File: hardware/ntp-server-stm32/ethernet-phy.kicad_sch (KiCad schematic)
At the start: 26 parts, among them U11 LAN8742AI-CZ-TR, Y1 25MHz

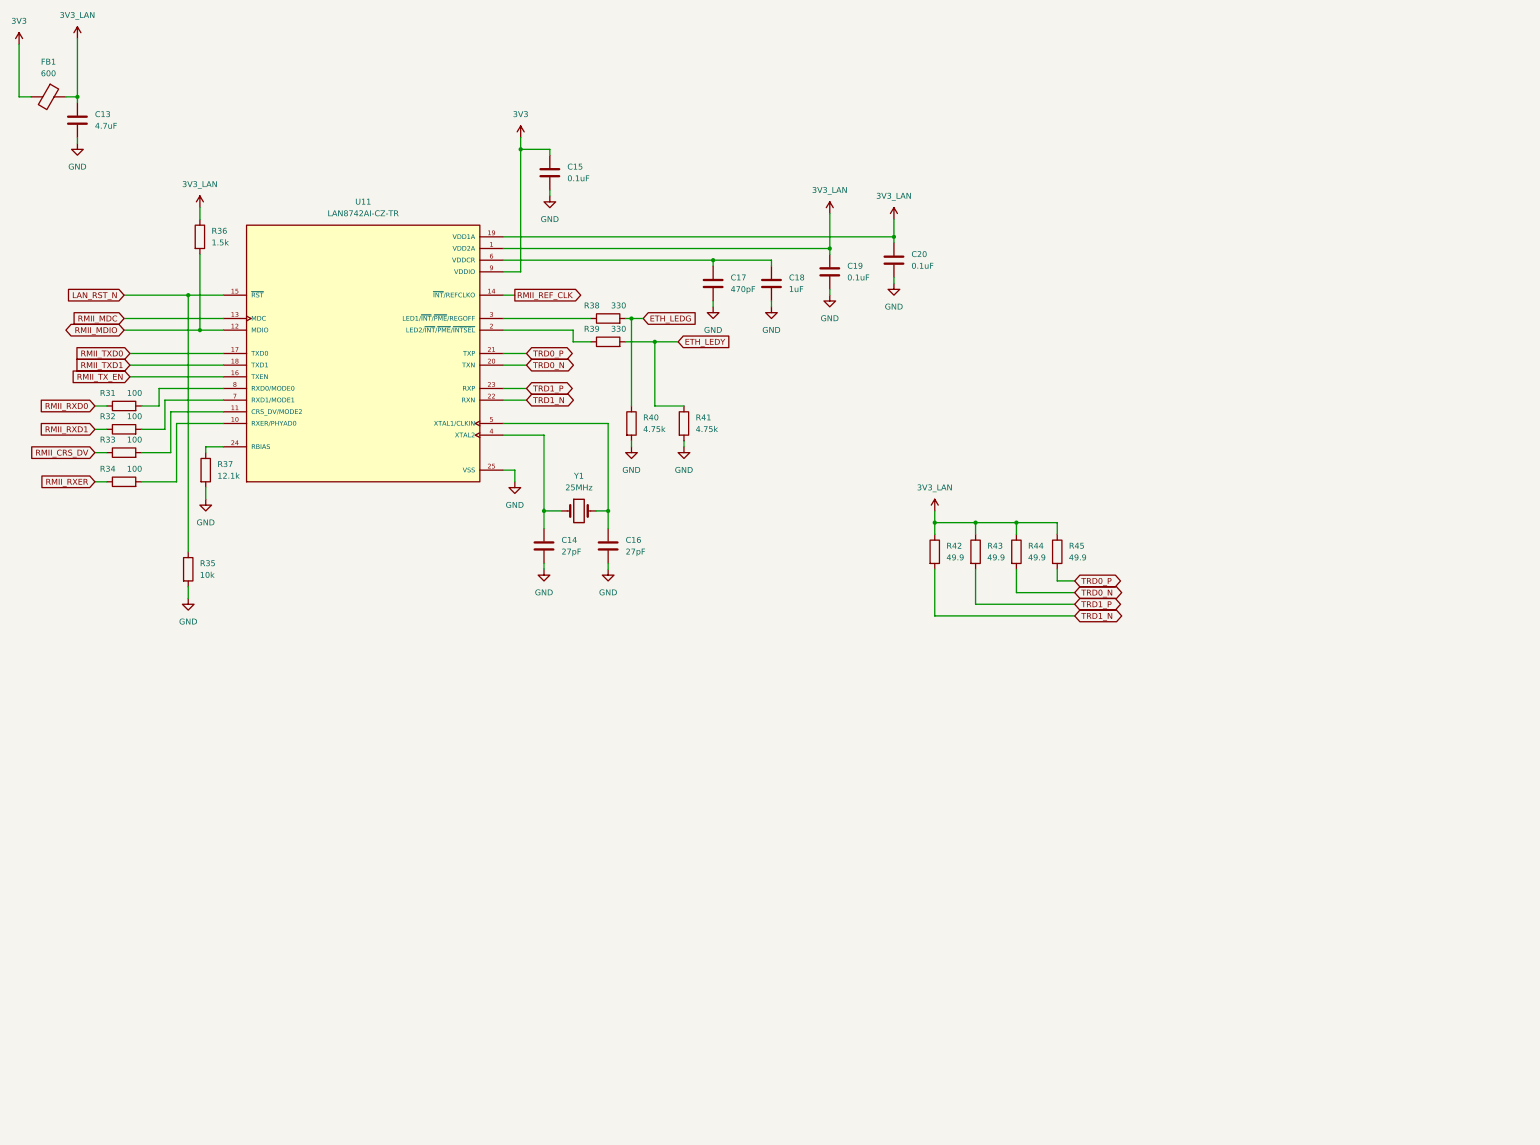
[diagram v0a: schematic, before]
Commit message: Updates
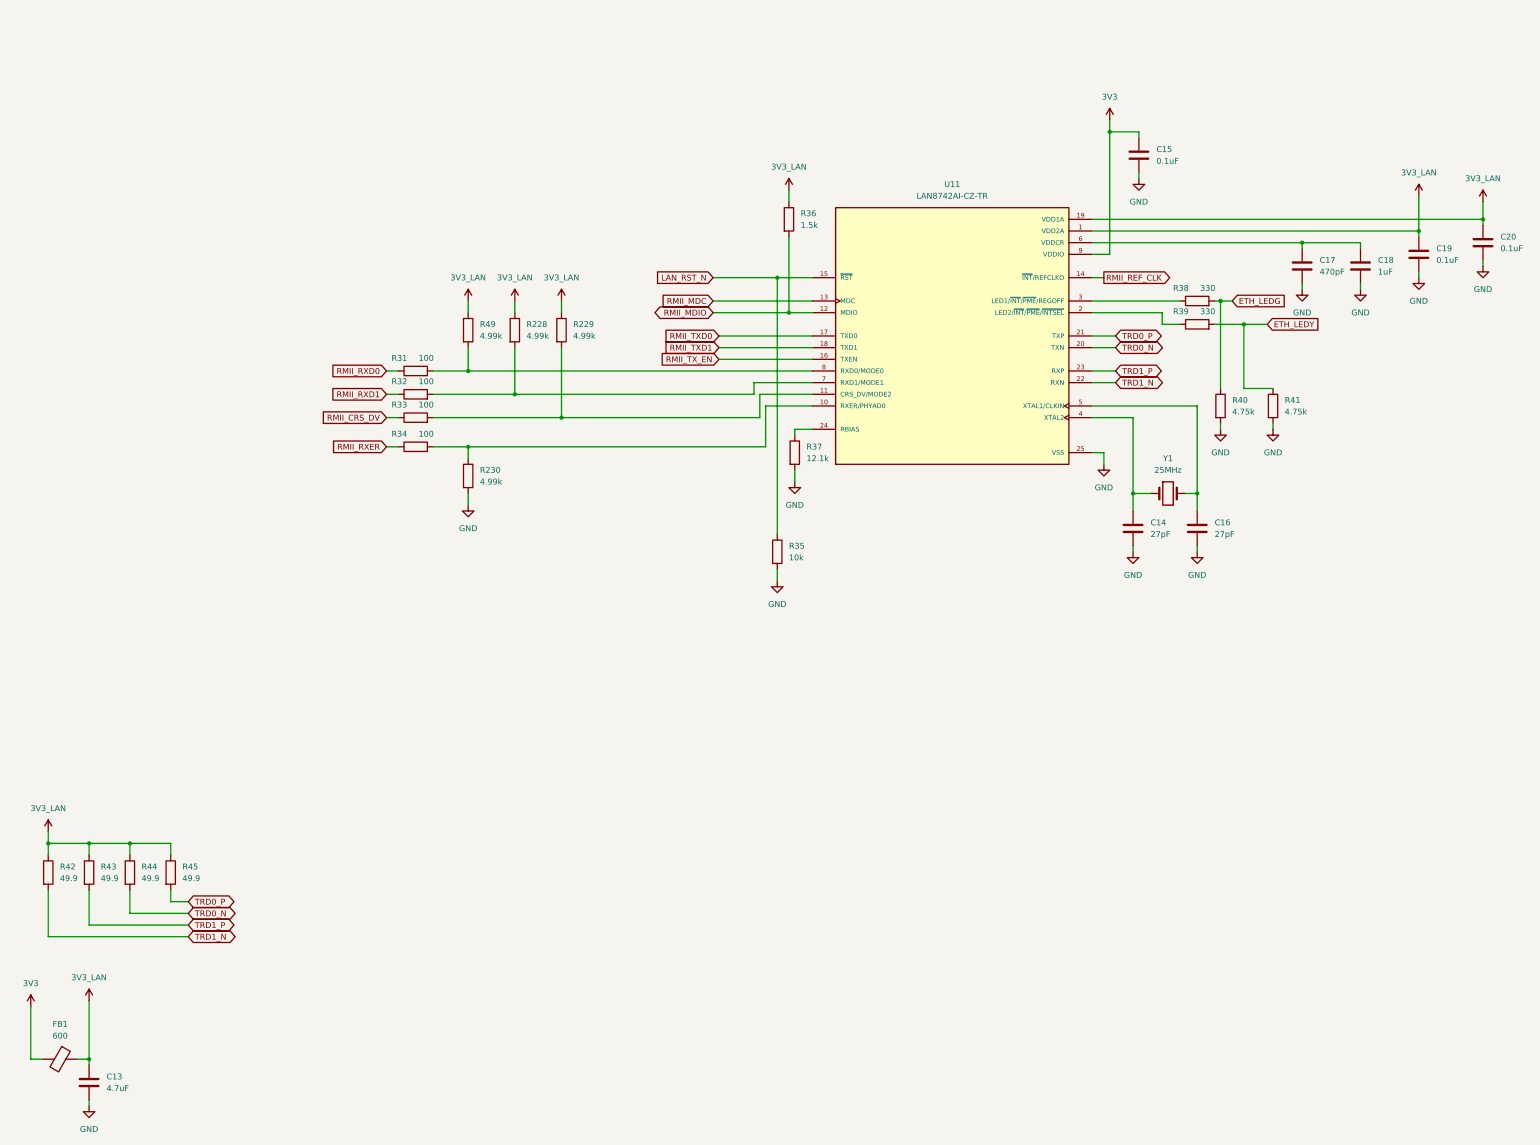
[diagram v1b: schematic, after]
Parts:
- added R228, R229, R230, R49: 4.99k, 0402 (1005 Metric), symbol Device:R
- C13: footprint C_0805_2012Metric -> 0805 (2012 Metric); DIELECTRIC (none) -> X7R; DIGIKEY_PART_NUMBER 490-GRM21BR71C475KE51KTR-ND -> 490-GRT21BR71C475KE13KCT-ND; MANUFACTURER Murata -> Murata Electronics; MANUFACTURER_PART_NUMBER GRM21BR71C475KE51K -> GRT21BR71C475KE13K; TOLERANCE (none) -> 10%; VOLTAGE (none) -> 16V
- C14, C16: footprint C_0402_1005Metric -> 0402 (1005 Metric); DIELECTRIC (none) -> C0G; DIGIKEY_PART_NUMBER (none) -> 490-12651-1-ND; MANUFACTURER (none) -> Murata Electronics; MANUFACTURER_PART_NUMBER (none) -> GCM1555C1H270JA16D; TOLERANCE (none) -> 5%; VOLTAGE (none) -> 50V
- C15, C19, C20: footprint C_0402_1005Metric -> 0402 (1005 Metric); DIELECTRIC (none) -> X7R; DIGIKEY_PART_NUMBER 490-6328-2-ND -> 490-4759-1-ND; MANUFACTURER_PART_NUMBER GRM155R71C104KA88J -> GCM155R71C104KA55D; TOLERANCE (none) -> 10%; VOLTAGE (none) -> 16V
- C17: footprint C_0402_1005Metric -> 0402 (1005 Metric); DIELECTRIC (none) -> C0G; DIGIKEY_PART_NUMBER (none) -> 490-GCM1555C1H471FA16DCT-ND; MANUFACTURER (none) -> Murata Electronics; MANUFACTURER_PART_NUMBER (none) -> GCM1555C1H471FA16D; TOLERANCE (none) -> 5%; VOLTAGE (none) -> 50V
- C18: footprint C_0603_1608Metric -> 0603 (1608 Metric); DIELECTRIC (none) -> X7R; DIGIKEY_PART_NUMBER (none) -> 399-17704-1-ND; MANUFACTURER (none) -> KEMET; MANUFACTURER_PART_NUMBER (none) -> C0603C105K4RACAUTO; TOLERANCE (none) -> 10%; VOLTAGE (none) -> 16V
- FB1: DIELECTRIC (none) -> Ferrite bead; MANUFACTURER Murata Electronics -> Murata; MANUFACTURER_PART_NUMBER BLM31KN601SN1L -> BLM31PG601SN1L; POWER (none) -> 3A
- R31, R32, R33, R34: footprint R_0402_1005Metric -> 0402 (1005 Metric); DIELECTRIC (none) -> Thick-film; DIGIKEY_PART_NUMBER (none) -> P100LCT-ND; MANUFACTURER Panasonic -> Panasonic Industry; POWER (none) -> 1/10W; TOLERANCE (none) -> 1%
- R35: footprint R_0402_1005Metric -> 0402 (1005 Metric); DIELECTRIC (none) -> Thick-film; DIGIKEY_PART_NUMBER (none) -> P10.0KLCT-ND; MANUFACTURER Panasonic -> Panasonic Industry; POWER (none) -> 1/10W; TOLERANCE (none) -> 1%
- R36: footprint R_0402_1005Metric -> 0402 (1005 Metric); DIELECTRIC (none) -> Thick-film; DIGIKEY_PART_NUMBER (none) -> P1.50KLCT-ND; MANUFACTURER Panasonic -> Panasonic Industry; POWER (none) -> 1/10W; TOLERANCE (none) -> 1%
- R37: footprint R_0402_1005Metric -> 0402 (1005 Metric); DIELECTRIC (none) -> Thick-film; DIGIKEY_PART_NUMBER (none) -> P12.1KLCT-ND; MANUFACTURER Panasonic -> Panasonic Industry; POWER (none) -> 1/10W; TOLERANCE (none) -> 1%
- R38, R39: footprint R_0402_1005Metric -> 0402 (1005 Metric); DIELECTRIC (none) -> Thick-film; DIGIKEY_PART_NUMBER (none) -> P330LCT-ND; MANUFACTURER Panasonic -> Panasonic Industry; POWER (none) -> 1/10W; TOLERANCE (none) -> 1%
- R40, R41: footprint R_0402_1005Metric -> 0402 (1005 Metric); DIELECTRIC (none) -> Thick-film; DIGIKEY_PART_NUMBER (none) -> 2019-RK73H1ERTTP4751FCT-ND; MANUFACTURER Panasonic -> KOA Speer Electronics, Inc.; MANUFACTURER_PART_NUMBER ERJ-2RKF4751X -> RK73H1ERTTP4751F; POWER (none) -> 1/10W; TOLERANCE (none) -> 1%
- R42, R43, R44, R45: footprint R_0402_1005Metric -> 0402 (1005 Metric); DIELECTRIC (none) -> Thick-film; DIGIKEY_PART_NUMBER (none) -> P49.9LCT-ND; MANUFACTURER Panasonic -> Panasonic Industry; POWER (none) -> 1/10W; TOLERANCE (none) -> 1%
- Y1: MANUFACTURER CTS-Frequency Controls -> CTS
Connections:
- net 3V3_LAN: now also R228.1, R229.1, R49.1
- net GND: now also R230.2
- net at R32.2, U11.7 (RXD1/MODE1): now also R228.2
- net at R33.2, U11.11 (CRS_DV/MODE2): now also R229.2
- net at R34.2, U11.10 (RXER/PHYAD0): now also R230.1
- net at R31.2, U11.8 (RXD0/MODE0): now also R49.2
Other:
- moved on the sheet: C13, C14, C15, C16, C17, C18, C19, C20, FB1, R31, R32, R33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

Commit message: Bom updates
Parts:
- FB1: footprint 1206 -> 1206 (3216 Metric)
- U11: DIGIKEY_PART_NUMBER (none) -> LAN8742AI-CZ-CT-ND
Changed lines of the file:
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@@
 			)
 		)
-		(property "Datasheet" ""
+		(property "Datasheet" "https://ww1.microchip.com/downloads/en/DeviceDoc/DS_LAN8742_00001989A.pdf"
 			(at 227.33 88.9 0)
 			(hide yes)
@@
 			)
 		)
-		(property "Description" "10/100 Ethernet PHY RMII QFN-24"
+		(property "Description" "IC TRANSCEIVER FULL 1/1 24SQFN"
 			(at 227.33 88.9 0)
 			(hide yes)
@@
 				)
 				(justify bottom)
+			)
+		)
+		(property "DIGIKEY_PART_NUMBER" "LAN8742AI-CZ-CT-ND"
+			(at 227.33 88.9 0)
+			(hide yes)
+			(show_name no)
+			(do_not_autoplace no)
+			(effects
+				(font
+					(size 1.27 1.27)
+				)
 			)
 		)
@@
 			)
 		)
-		(property "Footprint" "1206"
+		(property "Footprint" "1206 (3216 Metric)"
 			(at 33.02 244.602 90)
 			(hide yes)

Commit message: Add files via upload
Updated, completed placement
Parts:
- C13: footprint 0805 (2012 Metric) -> copy_ref:C_0805_2012Metric
- C14, C15, C16, C17, C19, C20: footprint 0402 (1005 Metric) -> copy_ref:C_0402_1005Metric
- C18: footprint 0603 (1608 Metric) -> copy_ref:C_0603_1608Metric
- FB1: footprint 1206 (3216 Metric) -> copy_ref:1206
- R228, R229, R230, R31, R32, R33, R34, R35, R36, R37, R38, R39, R40, R41, R42, R43, R44, R45, R49: footprint 0402 (1005 Metric) -> copy_ref:R_0402_1005Metric
- Y1: footprint (none) -> dowload:445I23E25M00000
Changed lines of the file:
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@@
 			)
 		)
-		(property "Footprint" "0402 (1005 Metric)"
+		(property "Footprint" "copy_ref:R_0402_1005Metric"
 			(at 110.49 103.378 90)
 			(hide yes)
@@
 			)
 		)
-		(property "Footprint" "0402 (1005 Metric)"
+		(property "Footprint" "copy_ref:R_0402_1005Metric"
 			(at 37.592 205.74 90)
 			(hide yes)
@@
 			)
 		)
-		(property "Footprint" "0402 (1005 Metric)"
+		(property "Footprint" "copy_ref:R_0402_1005Metric"
 			(at 28.702 205.74 90)
 			(hide yes)
@@
 			)
 		)
-		(property "Footprint" "0402 (1005 Metric)"
+		(property "Footprint" "copy_ref:R_0402_1005Metric"
 			(at 280.67 83.058 90)
 			(hide yes)
@@
 			)
 		)
-		(property "Footprint" "0402 (1005 Metric)"
+		(property "Footprint" "copy_ref:C_0402_1005Metric"
 			(at 329.8952 74.93 0)
 			(hide yes)
@@
 			)
 		)
-		(property "Footprint" "0402 (1005 Metric)"
+		(property "Footprint" "copy_ref:R_0402_1005Metric"
 			(at 280.67 88.138 90)
 			(hide yes)
@@
 			)
 		)
-		(property "Footprint" "0402 (1005 Metric)"
+		(property "Footprint" "copy_ref:C_0402_1005Metric"
 			(at 268.9352 53.34 0)
 			(hide yes)
@@
 			)
 		)
-		(property "Footprint" "0402 (1005 Metric)"
+		(property "Footprint" "copy_ref:R_0402_1005Metric"
 			(at 55.372 205.74 90)
 			(hide yes)
@@
 			)
 		)
-		(property "Footprint" "0402 (1005 Metric)"
+		(property "Footprint" "copy_ref:C_0402_1005Metric"
 			(at 281.6352 134.62 0)
 			(hide yes)
@@
 			)
 		)
-		(property "Footprint" "0402 (1005 Metric)"
+		(property "Footprint" "copy_ref:C_0402_1005Metric"
 			(at 304.4952 77.47 0)
 			(hide yes)
@@
 			)
 		)
-		(property "Footprint" "0402 (1005 Metric)"
+		(property "Footprint" "copy_ref:R_0402_1005Metric"
 			(at 110.49 108.458 90)
 			(hide yes)
@@
 			)
 		)
-		(property "Footprint" "0402 (1005 Metric)"
+		(property "Footprint" "copy_ref:R_0402_1005Metric"
 			(at 120.142 87.63 90)
 			(hide yes)
@@
 			)
 		)
-		(property "Footprint" "0402 (1005 Metric)"
+		(property "Footprint" "copy_ref:C_0402_1005Metric"
 			(at 267.6652 134.62 0)
 			(hide yes)
@@
 			)
 		)
-		(property "Footprint" "0402 (1005 Metric)"
+		(property "Footprint" "copy_ref:R_0402_1005Metric"
 			(at 283.972 104.14 90)
 			(hide yes)
@@
 			)
 		)
-		(property "Footprint" "0402 (1005 Metric)"
+		(property "Footprint" "copy_ref:R_0402_1005Metric"
 			(at 120.142 119.38 90)
 			(hide yes)
@@
 			)
 		)
-		(property "Footprint" "0402 (1005 Metric)"
+		(property "Footprint" "copy_ref:R_0402_1005Metric"
 			(at 295.402 104.14 90)
 			(hide yes)
@@
 			)
 		)
-		(property "Footprint" "0402 (1005 Metric)"
+		(property "Footprint" "copy_ref:R_0402_1005Metric"
 			(at 191.262 114.3 90)
 			(hide yes)
@@
 			)
 		)
-		(property "Footprint" "0402 (1005 Metric)"
+		(property "Footprint" "copy_ref:R_0402_1005Metric"
 			(at 130.302 87.63 90)
 			(hide yes)
@@
 			)
 		)
-		(property "Footprint" "0402 (1005 Metric)"
+		(property "Footprint" "copy_ref:C_0402_1005Metric"
 			(at 343.8652 72.39 0)
 			(hide yes)
@@
 			)
 		)
-		(property "Footprint" "0603 (1608 Metric)"
+		(property "Footprint" "copy_ref:C_0603_1608Metric"
 			(at 317.1952 77.47 0)
 			(hide yes)
@@
 			)
 		)
-		(property "Footprint" "0402 (1005 Metric)"
+		(property "Footprint" "copy_ref:R_0402_1005Metric"
 			(at 110.49 114.808 90)
 			(hide yes)
@@
 			)
 		)
-		(property "Footprint" ""
+		(property "Footprint" "dowload:445I23E25M00000"
 			(at 274.32 123.19 0)
 			(hide yes)
@@
 			)
 		)
-		(property "Footprint" "0402 (1005 Metric)"
+		(property "Footprint" "copy_ref:R_0402_1005Metric"
 			(at 189.992 63.5 90)
 			(hide yes)
@@
 			)
 		)
-		(property "Footprint" "0402 (1005 Metric)"
+		(property "Footprint" "copy_ref:R_0402_1005Metric"
 			(at 187.452 135.89 90)
 			(hide yes)
@@
 			)
 		)
-		(property "Footprint" "1206 (3216 Metric)"
+		(property "Footprint" "copy_ref:1206"
 			(at 33.02 244.602 90)
 			(hide yes)
@@
 			)
 		)
-		(property "Footprint" "0805 (2012 Metric)"
+		(property "Footprint" "copy_ref:C_0805_2012Metric"
 			(at 40.3352 255.27 0)
 			(hide yes)
@@
 			)
 		)
-		(property "Footprint" "0402 (1005 Metric)"
+		(property "Footprint" "copy_ref:R_0402_1005Metric"
 			(at 110.49 98.298 90)
 			(hide yes)
@@
 			)
 		)
-		(property "Footprint" "0402 (1005 Metric)"
+		(property "Footprint" "copy_ref:R_0402_1005Metric"
 			(at 140.462 87.63 90)
 			(hide yes)
@@
 			)
 		)
-		(property "Footprint" "0402 (1005 Metric)"
+		(property "Footprint" "copy_ref:R_0402_1005Metric"
 			(at 46.482 205.74 90)
 			(hide yes)
